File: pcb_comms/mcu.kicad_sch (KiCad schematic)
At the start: 33 parts, among them SW1 SW_SPDT, U3 STM32WLE5CCU6, Y1 32.768KHz, Y2 32MHz

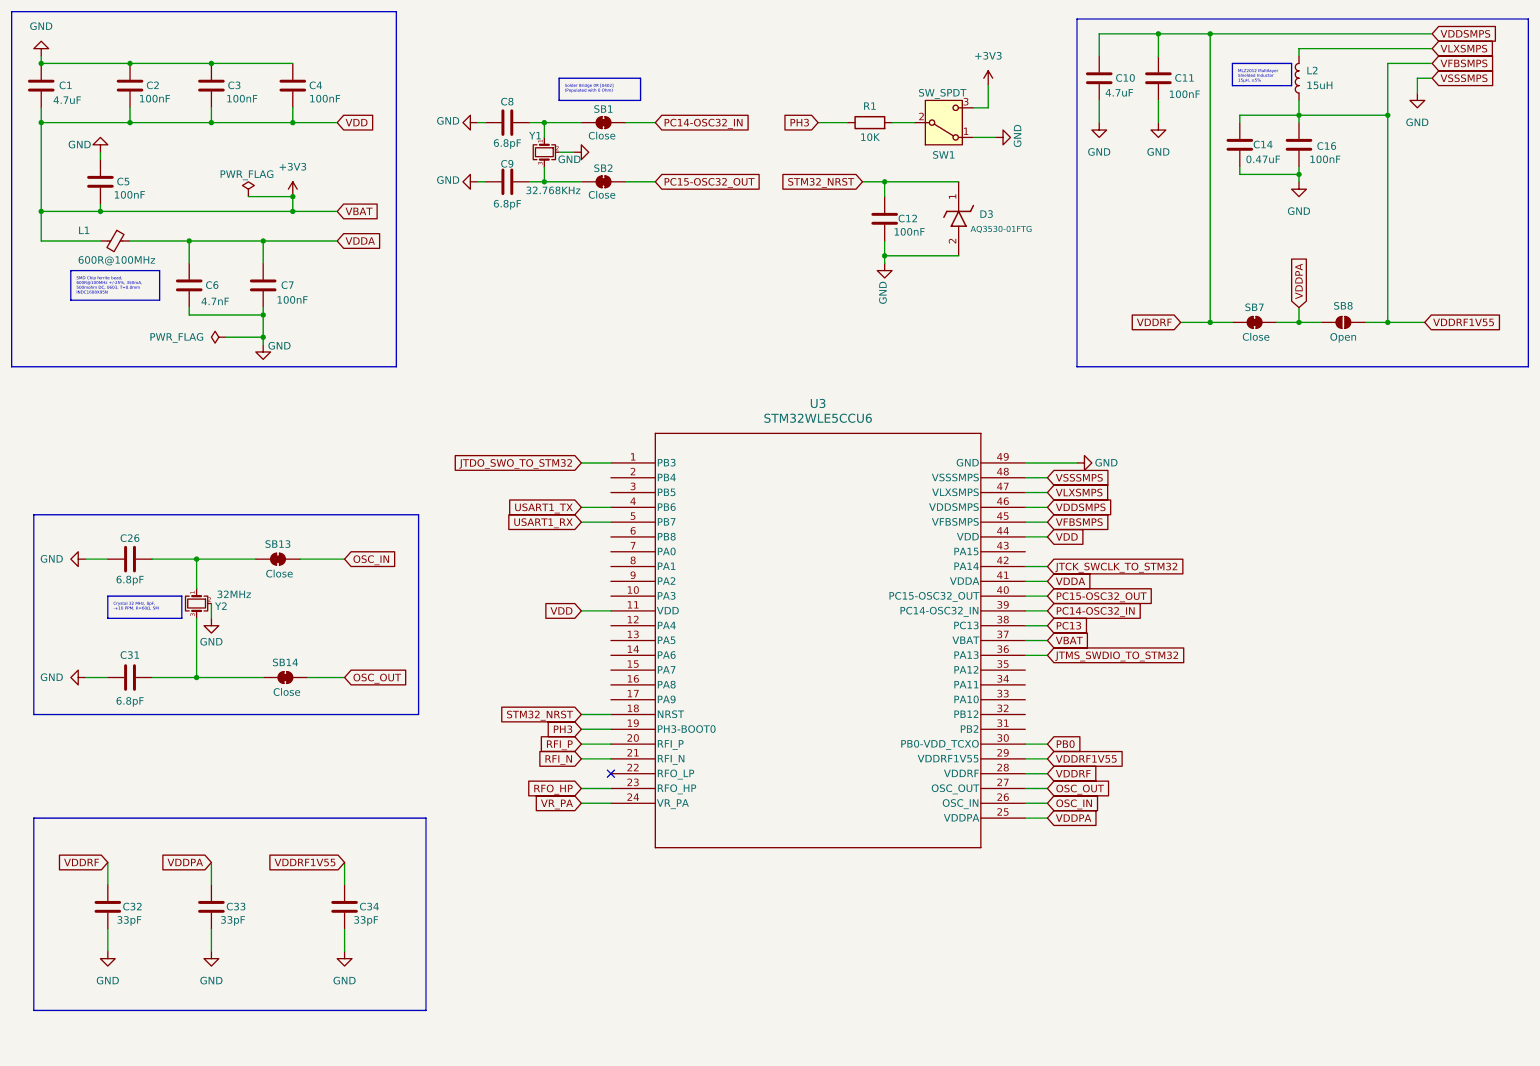
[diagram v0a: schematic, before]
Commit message: Update GPS
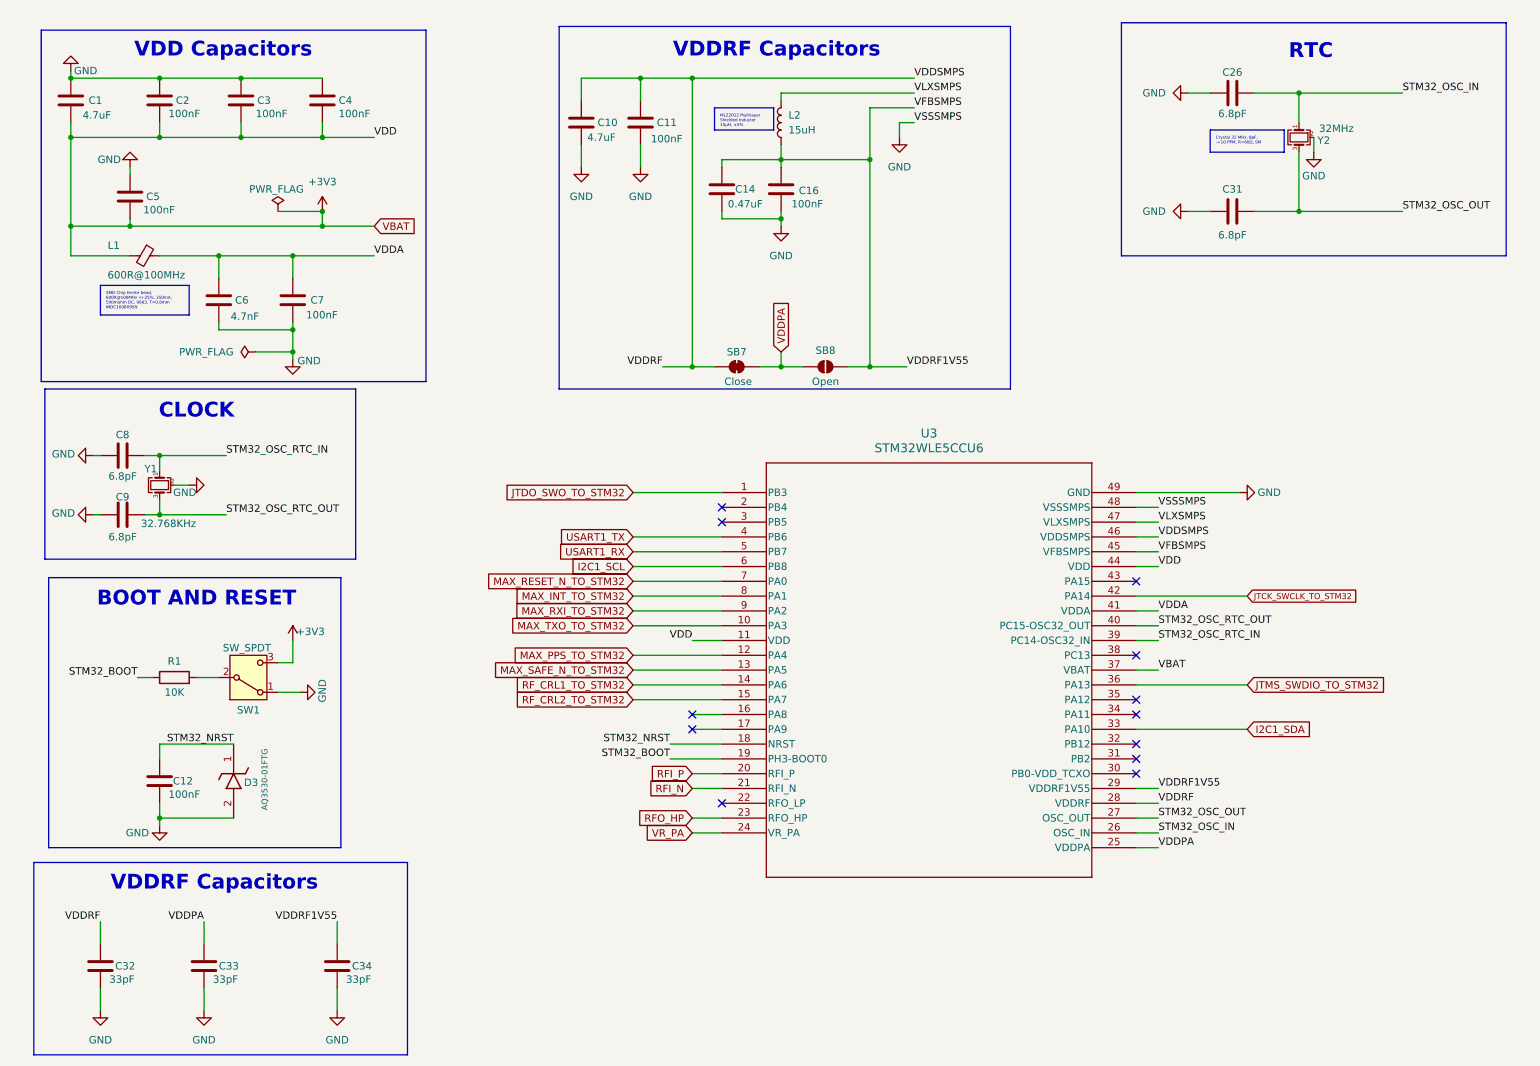
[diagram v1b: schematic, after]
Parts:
- removed SB1, SB13, SB14, SB2: Close, symbol Jumper:SolderJumper_2_Bridged
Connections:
- net OSC_IN is gone; now on net STM32_OSC_IN: U3.26 (OSC_IN)
- net OSC_OUT is gone; now on net STM32_OSC_OUT: U3.27 (OSC_OUT)
- net PC14-OSC32_IN is gone; now on net STM32_OSC_RTC_IN: U3.39 (PC14-OSC32_IN)
- net PC15-OSC32_OUT is gone; now on net STM32_OSC_RTC_OUT: U3.40 (PC15-OSC32_OUT)
- net STM32_OSC_IN: now reaches C26.2, Y2.1
- net MAX_TXO_TO_STM32: now reaches U3.10 (PA3)
- net MAX_PPS_TO_STM32: now reaches U3.12 (PA4)
- net MAX_SAFE_N_TO_STM32: now reaches U3.13 (PA5)
- net RF_CRL1_TO_STM32: now reaches U3.14 (PA6)
- net RF_CRL2_TO_STM32: now reaches U3.15 (PA7)
- net I2C1_SDA: now reaches U3.33 (PA10)
- net I2C1_SCL: now reaches U3.6 (PB8)
- net MAX_RESET_N_TO_STM32: now reaches U3.7 (PA0)
- net MAX_INT_TO_STM32: now reaches U3.8 (PA1)
- net MAX_RXI_TO_STM32: now reaches U3.9 (PA2)
- net STM32_OSC_RTC_OUT: now reaches C9.2, Y1.3
- net STM32_OSC_OUT: now reaches C31.2, Y2.3
- net STM32_OSC_RTC_IN: now reaches C8.2, Y1.1
- net PB0: no longer names the net of U3.30 (PB0-VDD_TCXO)
- net PC13: no longer names the net of U3.38 (PC13)
- net PH3 renamed STM32_BOOT
- no-connect marks 1 -> 12
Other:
- note added: "BOOT AND RESET"
- note added: "CLOCK"
- note added: "RTC"
- note added: "VDD Capacitors"
- note added: "VDDRF Capacitors"
- moved on the sheet: C1, C10, C11, C12, C14, C16, C2, C26, C3, C31, C32, C33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
